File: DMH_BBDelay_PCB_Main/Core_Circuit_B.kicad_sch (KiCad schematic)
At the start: 73 parts, among them Q8 J113, SW1 SW_DPDT_3way_x2, SW2 SW_DPDT_x2, SW4 SW_SPDT, U18 CD4053B, U5 TL074, U6 TL074, U7 V3205, U8 CD4046, U9 40106

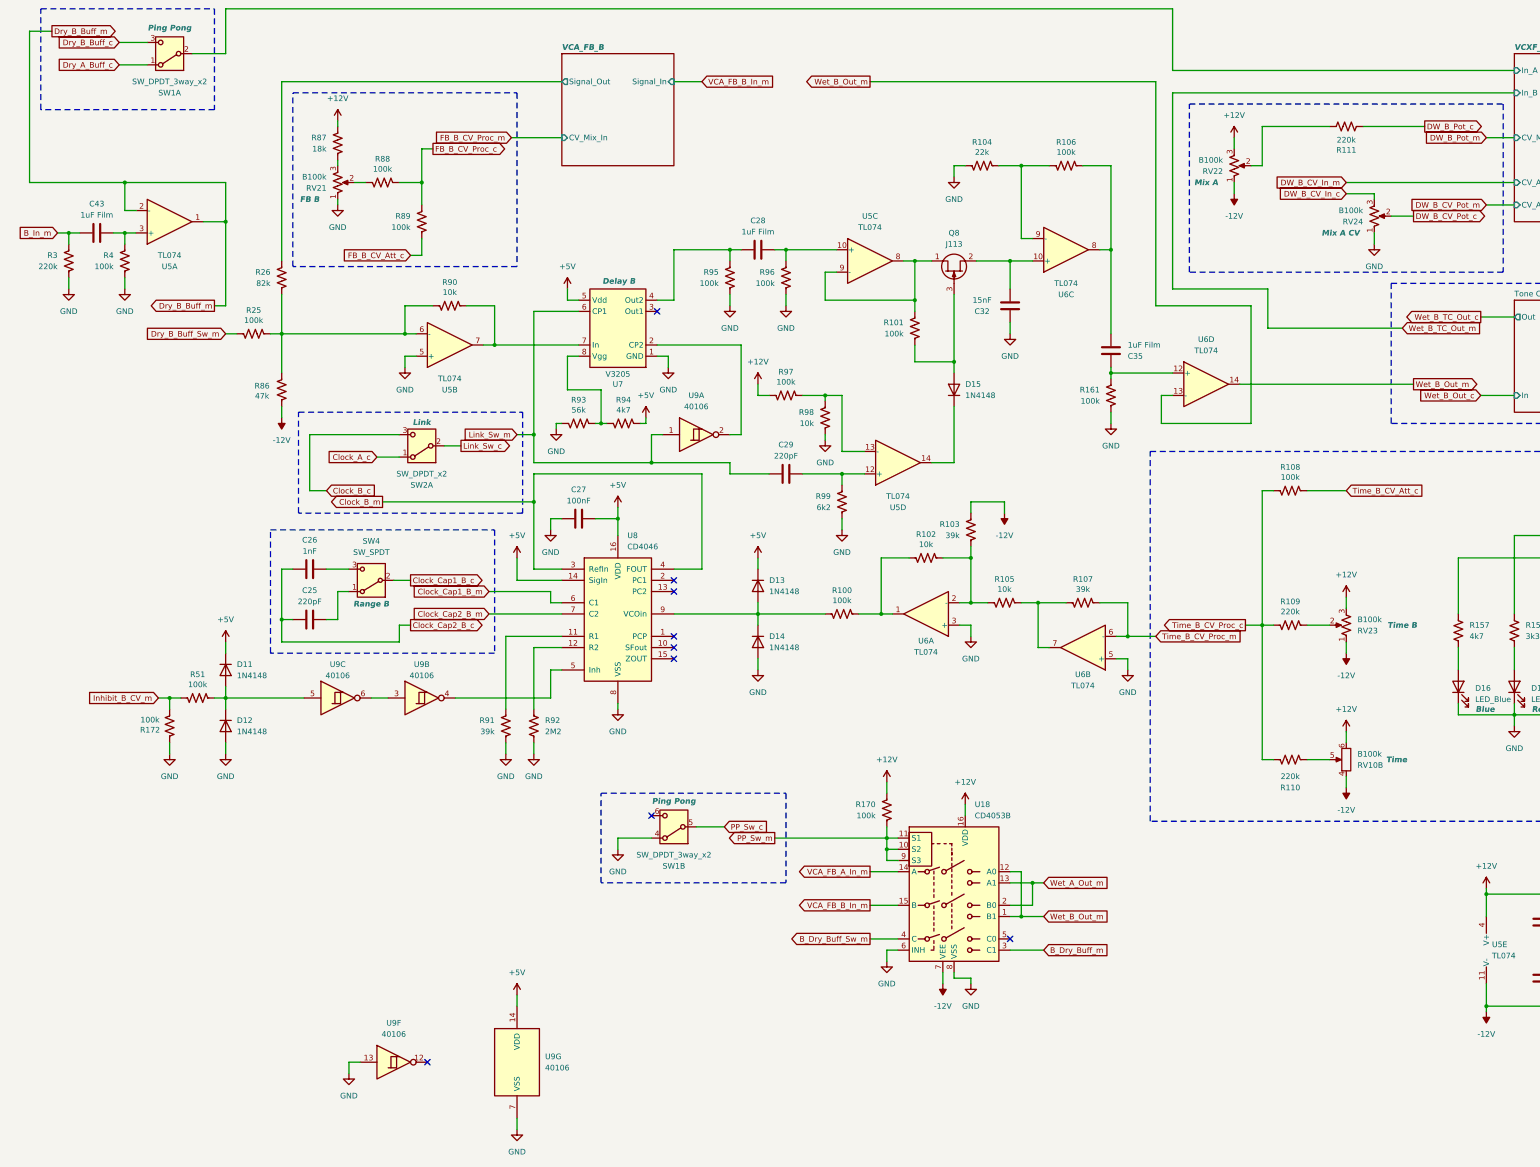
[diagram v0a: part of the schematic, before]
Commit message: Schematic ready for breadboarding
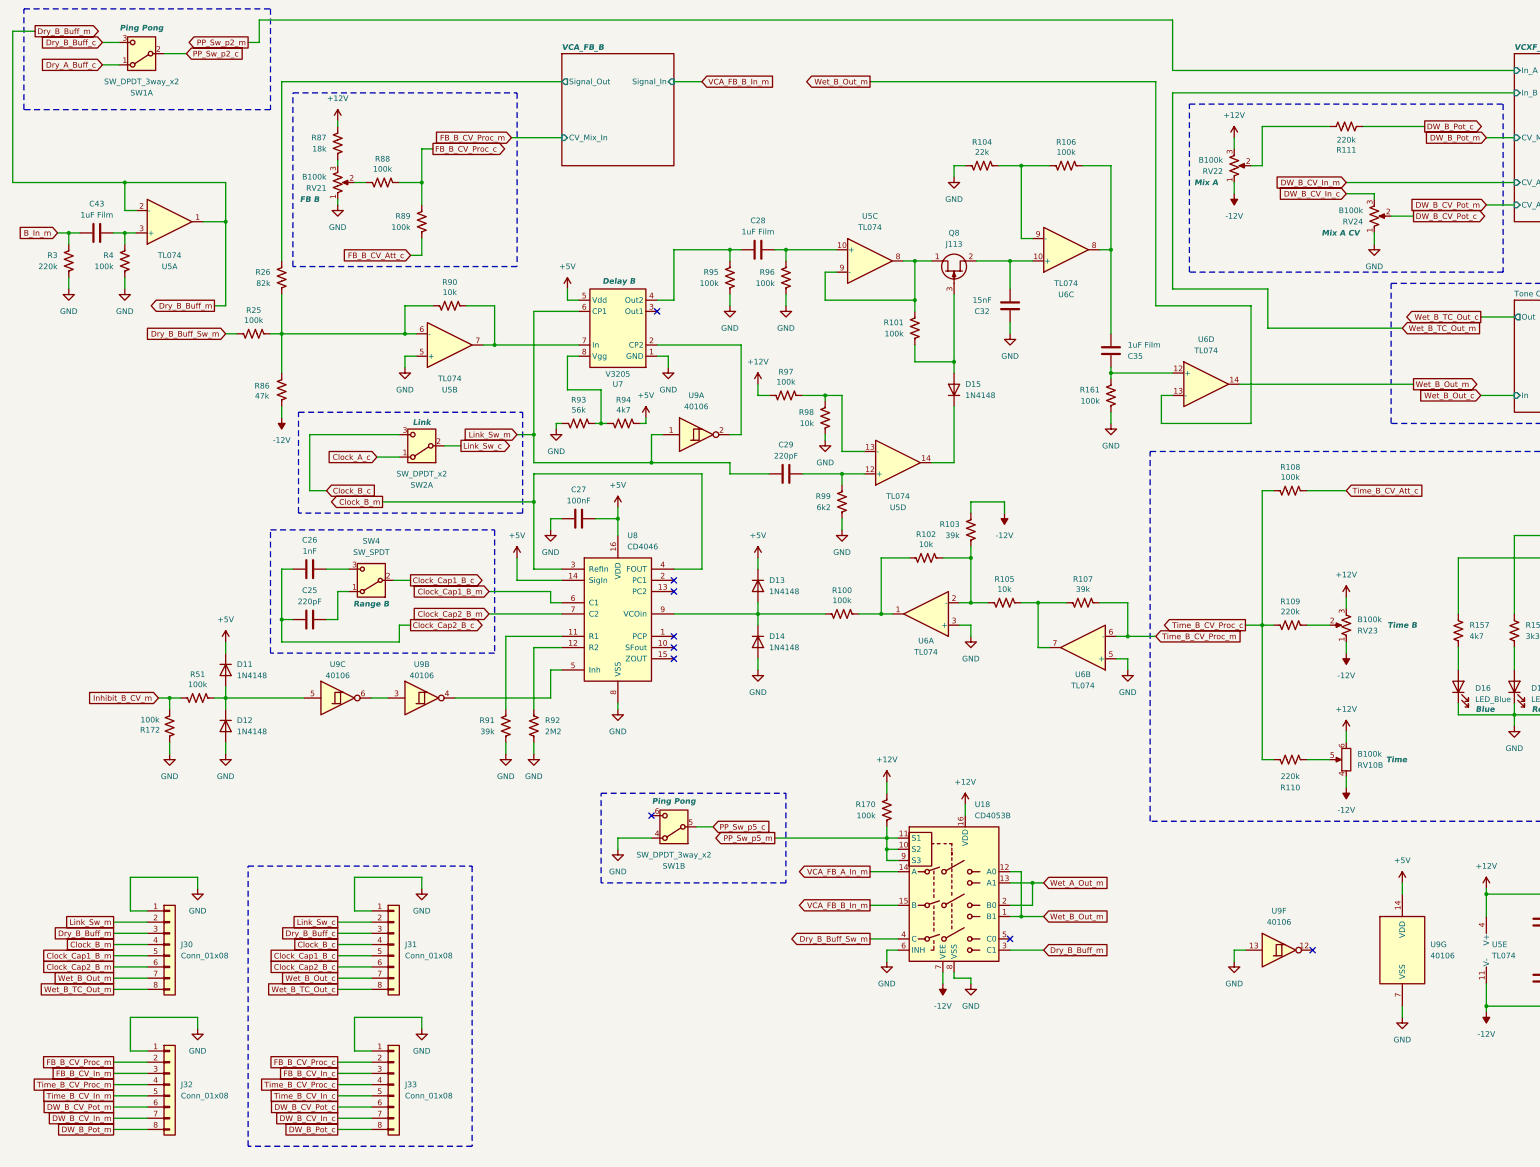
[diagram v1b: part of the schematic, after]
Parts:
- added J30, J32: Conn_01x08, Connector_PinHeader_2.54mm:PinHeader_1x08_P2.54mm_Vertical, symbol Connector_Generic:Conn_01x08
- added J31, J33: Conn_01x08, Connector_PinSocket_2.54mm:PinSocket_1x08_P2.54mm_Vertical, symbol Connector_Generic:Conn_01x08
- SW1, SW2: footprint (none) -> SynthStuff:Toggle_Switch_2_Poles_TE
- SW4: footprint (none) -> SynthStuff:Toggle_Switch_TE
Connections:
- net B_Dry_Buff_Sw_m is gone; now on net Dry_B_Buff_Sw_m: U18.4 (C)
- net B_Dry_Buff_m is gone; now on net Dry_B_Buff_m: U18.3 (C1)
- net Clock_B_c: now also J31.4 (Pin_4)
- net Clock_B_m: now also J30.4 (Pin_4)
- net Clock_Cap1_B_c: now also J31.5 (Pin_5)
- net Clock_Cap1_B_m: now also J30.5 (Pin_5)
- net Clock_Cap2_B_c: now also J31.6 (Pin_6)
- net Clock_Cap2_B_m: now also J30.6 (Pin_6)
- net DW_B_CV_In_c: now also J33.7 (Pin_7)
- net DW_B_CV_In_m: now also J32.7 (Pin_7)
- net DW_B_CV_Pot_c: now also J33.6 (Pin_6)
- net DW_B_CV_Pot_m: now also J32.6 (Pin_6)
- net DW_B_Pot_c: now also J33.8 (Pin_8)
- net DW_B_Pot_m: now also J32.8 (Pin_8)
- net Dry_B_Buff_c: now also J31.3 (Pin_3)
- net Dry_B_Buff_m: now also J30.3 (Pin_3)
- net FB_B_CV_Proc_c: now also J33.2 (Pin_2)
- net FB_B_CV_Proc_m: now also J32.2 (Pin_2)
- net GND: now also J30.1 (Pin_1), J31.1 (Pin_1), J32.1 (Pin_1), J33.1 (Pin_1)
- net Link_Sw_c: now also J31.2 (Pin_2)
- net Link_Sw_m: now also J30.2 (Pin_2)
- net Time_B_CV_Proc_c: now also J33.4 (Pin_4)
- net Time_B_CV_Proc_m: now also J32.4 (Pin_4)
- net Wet_B_Out_c: now also J31.7 (Pin_7)
- net Wet_B_Out_m: now also J30.7 (Pin_7)
- net Wet_B_TC_Out_c: now also J31.8 (Pin_8)
- net Wet_B_TC_Out_m: now also J30.8 (Pin_8)
- net PP_Sw_c renamed PP_Sw_p5_c
- net PP_Sw_m renamed PP_Sw_p5_m
- net VCXF_DW_B/In_A renamed PP_Sw_p2_c
- new net FB_B_CV_In_c: J33.3 (Pin_3)
- new net FB_B_CV_In_m: J32.3 (Pin_3)
- new net Time_B_CV_In_c: J33.5 (Pin_5)
- new net Time_B_CV_In_m: J32.5 (Pin_5)
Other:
- moved on the sheet: SW1A, U9F, U9G
